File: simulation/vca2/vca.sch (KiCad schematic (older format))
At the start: 34 parts, among them Q1 BC557B, Q2 BC557B, Q3 BC557B, Q4 BC557B, Q6 BC557B, Q8 BC557B, U1 LM324, U2 LM324

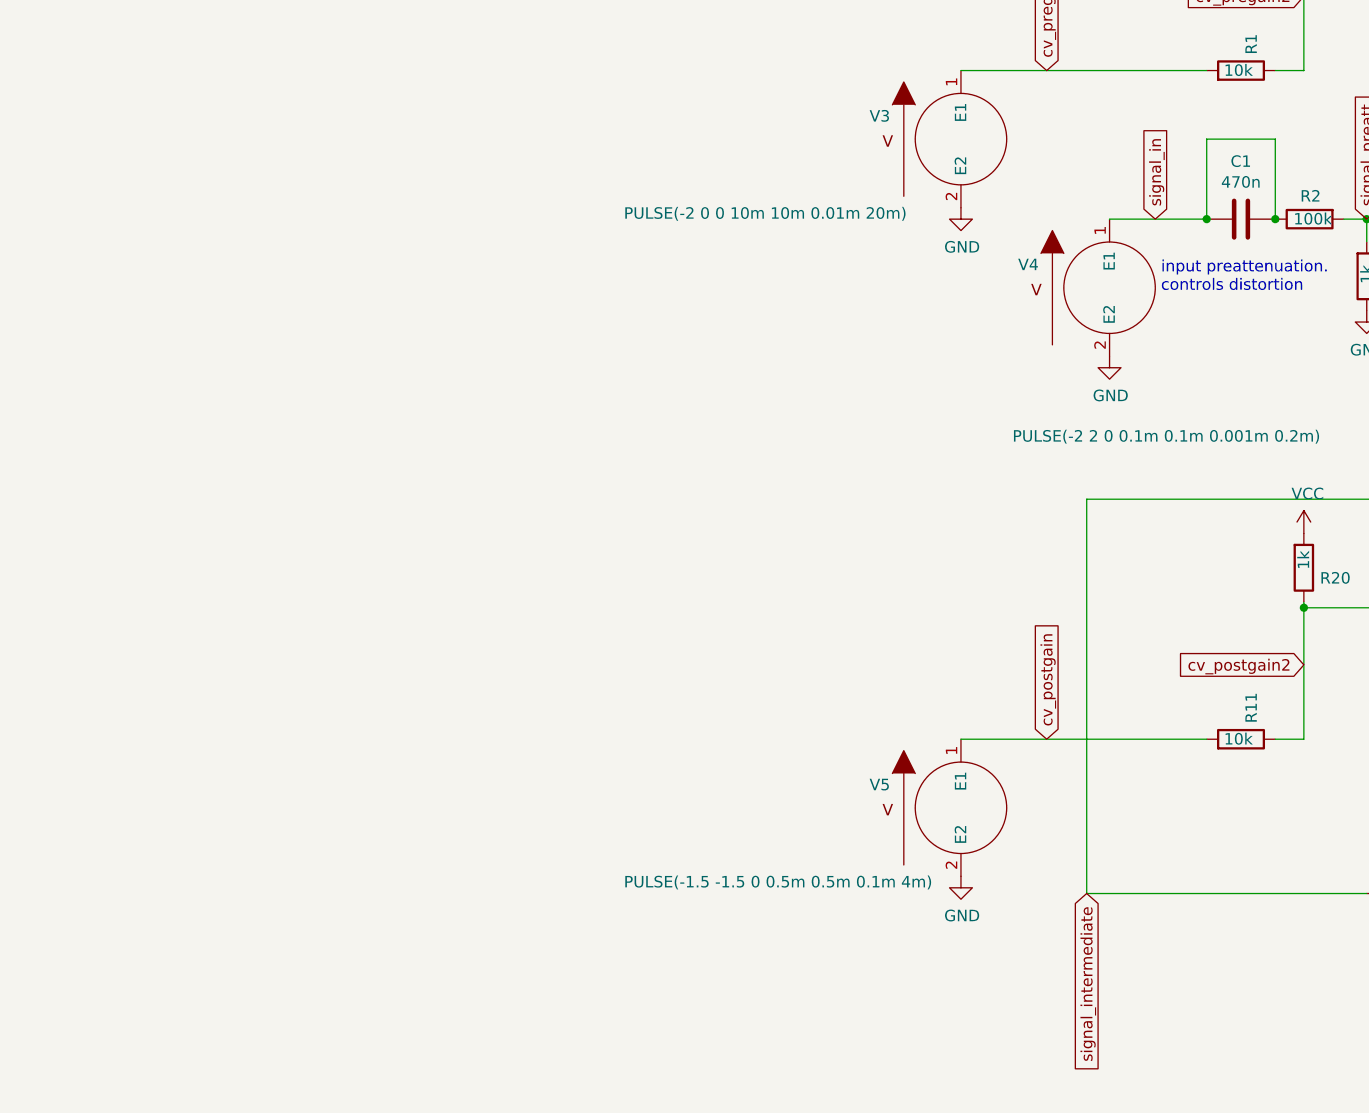
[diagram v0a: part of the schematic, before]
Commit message: vca with voltage controlled distortion that does not affect volume
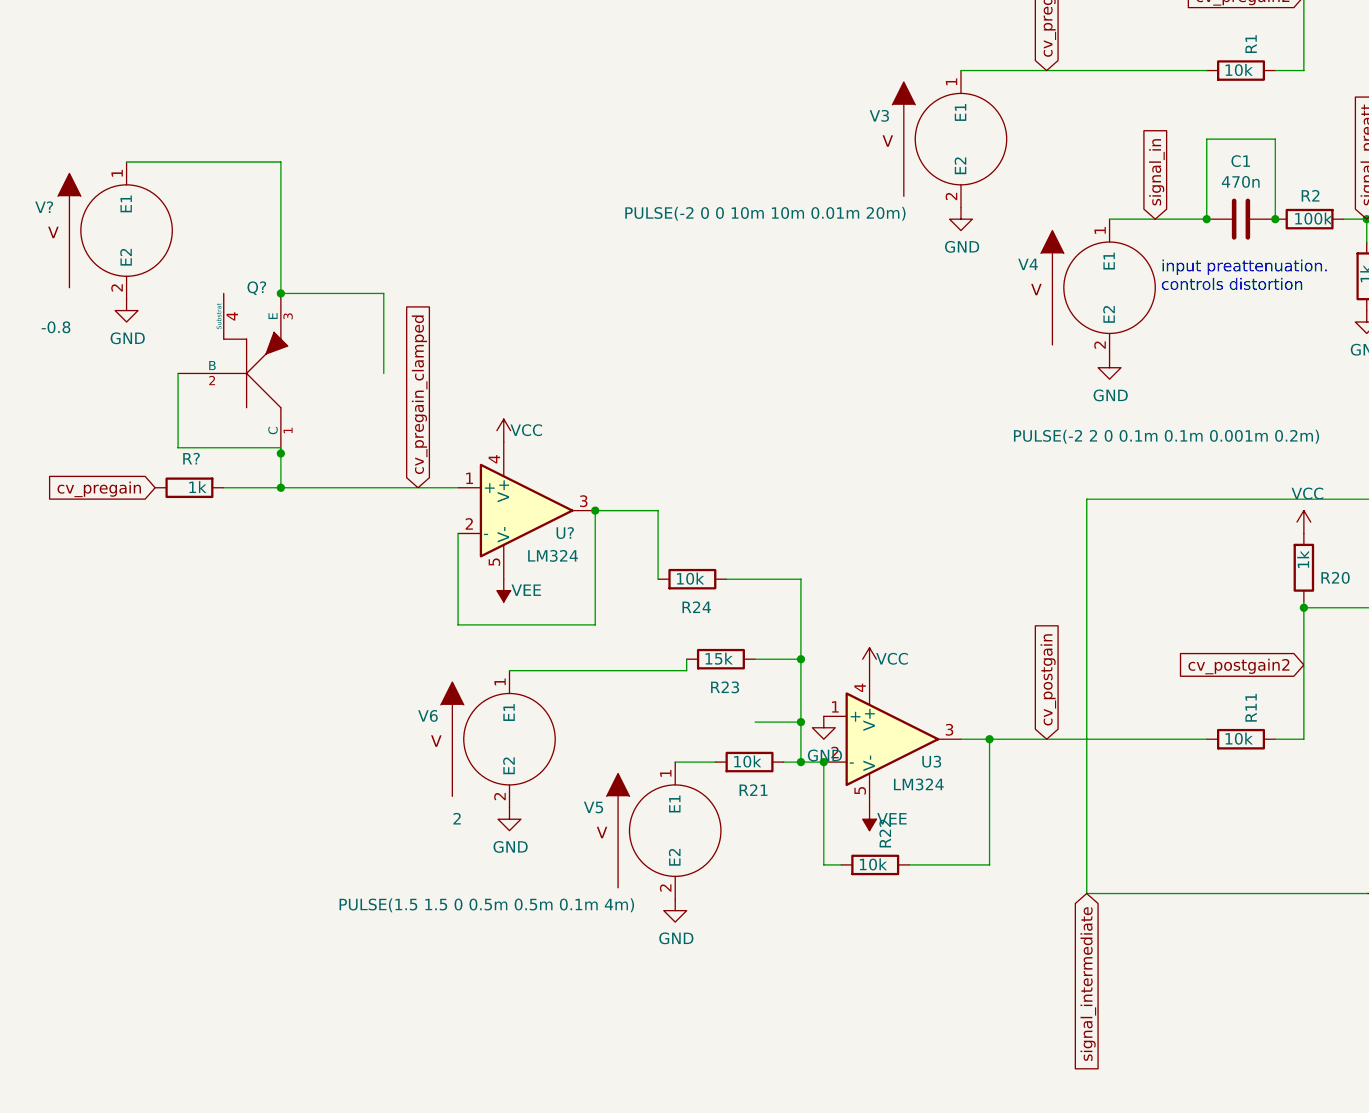
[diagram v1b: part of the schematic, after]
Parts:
- added Q?: BC557B, symbol pspice:QPNP
- added R21, R22, R24: 10k, symbol Device:R
- added R23: 15k, symbol Device:R
- added R?: 1k, symbol Device:R
- added U3, U?: LM324, symbol pspice:OPAMP
- added V6: 2, symbol pspice:VSOURCE
- added V?: -0.8, symbol pspice:VSOURCE
- V5: value PULSE(-1.5 -1.5 0 0.5m 0.5m 0.1m 4m) -> PULSE(1.5 1.5 0 0.5m 0.5m 0.1m 4m)
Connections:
- net 0: now also U3.1 (+), V6.2 (E2), V?.2 (E2)
- net VCC: now also U3.4 (V+), U?.4 (V+)
- net VEE: now also U3.5 (V-), U?.5 (V-)
- net cv_postgain: now also R22.1, U3.3; no longer V5.1 (E1)
- net cv_pregain: now also R?.1
- new net: R21.2, V5.1 (E1)
- new net: R21.1, R22.2, R23.1, R24.1, U3.2 (-)
- new net: R24.2, U?.2 (-), U?.3
- new net: R23.2, V6.1 (E1)
- new net: Q?.3 (E), V?.1 (E1)
- new net cv_pregain_clamped: Q?.1 (C), Q?.2 (B), R?.2, U?.1 (+)
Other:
- moved on the sheet: V5
